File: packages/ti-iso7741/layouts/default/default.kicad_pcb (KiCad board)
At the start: 2 copper layers, 5 parts

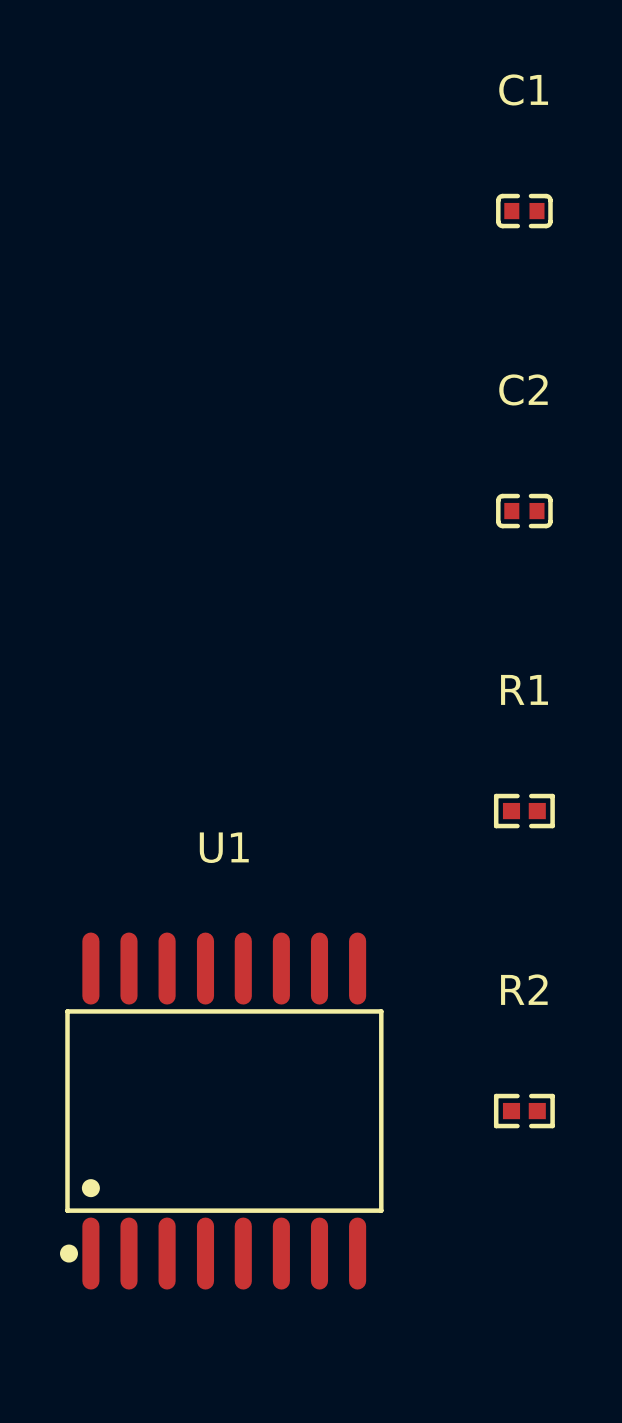
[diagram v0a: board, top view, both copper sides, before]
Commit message: Layout modules
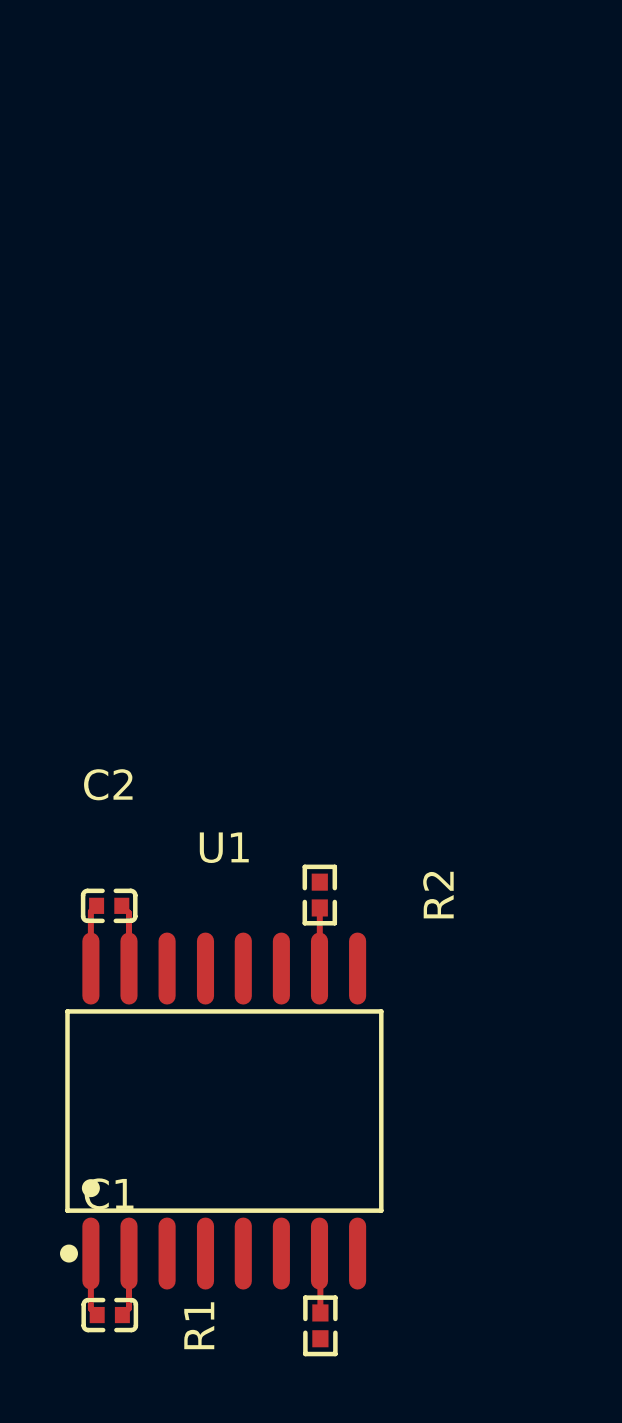
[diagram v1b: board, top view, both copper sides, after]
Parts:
- moved C1 39.3 mm to (-3.82, 6.80)
- moved C2 19.1 mm to (-3.84, -6.84)
- moved R1 18.5 mm to (3.20, 7.16), turned to 90 degrees
- moved R2 9.92 mm to (3.18, -7.20), turned to -90 degrees
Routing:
- net decap_side2-power-lv: track 0.00 -> 2.19 mm
- net decap_side2-power-hv: track 0.00 -> 2.17 mm
- net lv: track 0.00 -> 2.14 mm
- net hv: track 0.00 -> 2.14 mm
- net 10: track 0.00 -> 2.02 mm
- net 7: track 0.00 -> 1.99 mm
